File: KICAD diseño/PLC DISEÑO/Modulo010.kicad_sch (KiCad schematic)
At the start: 8 parts

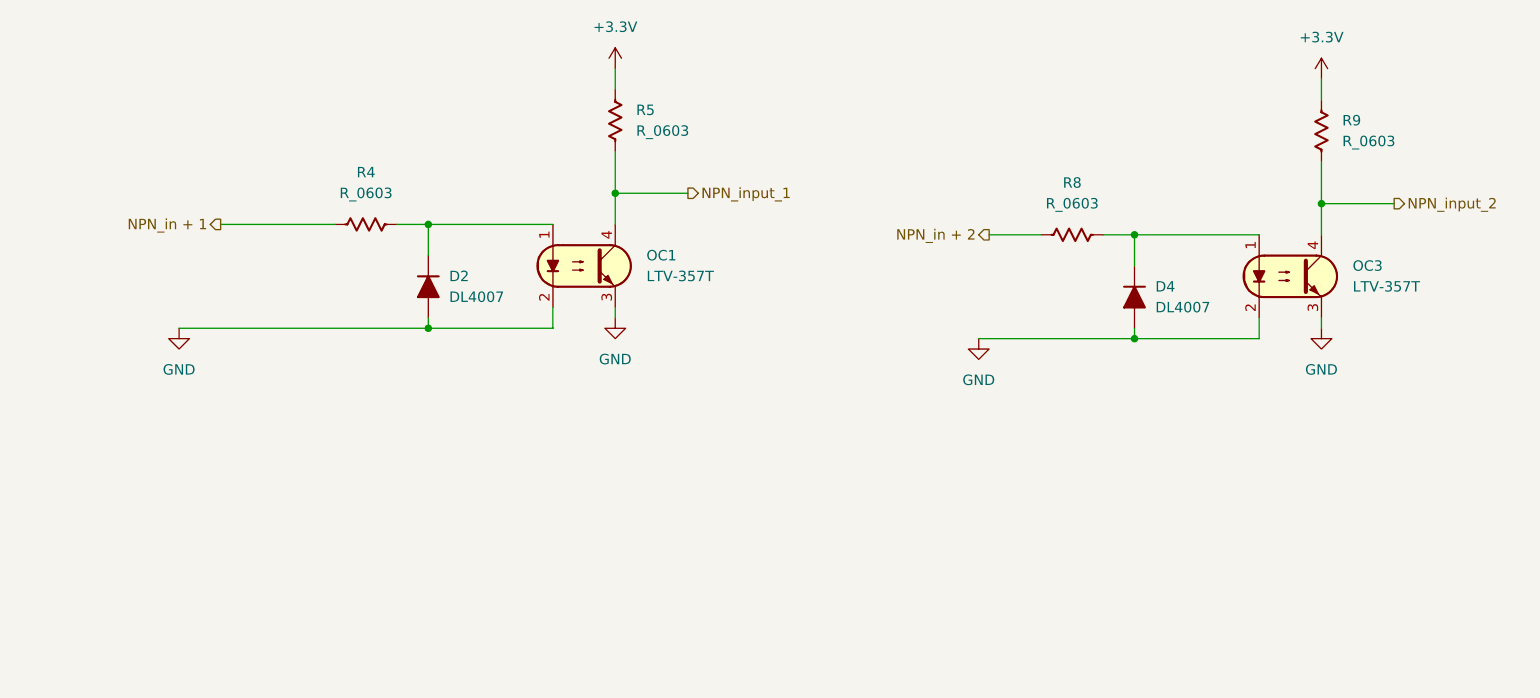
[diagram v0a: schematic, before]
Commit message: Actualizacion estoy cansado jefe :)
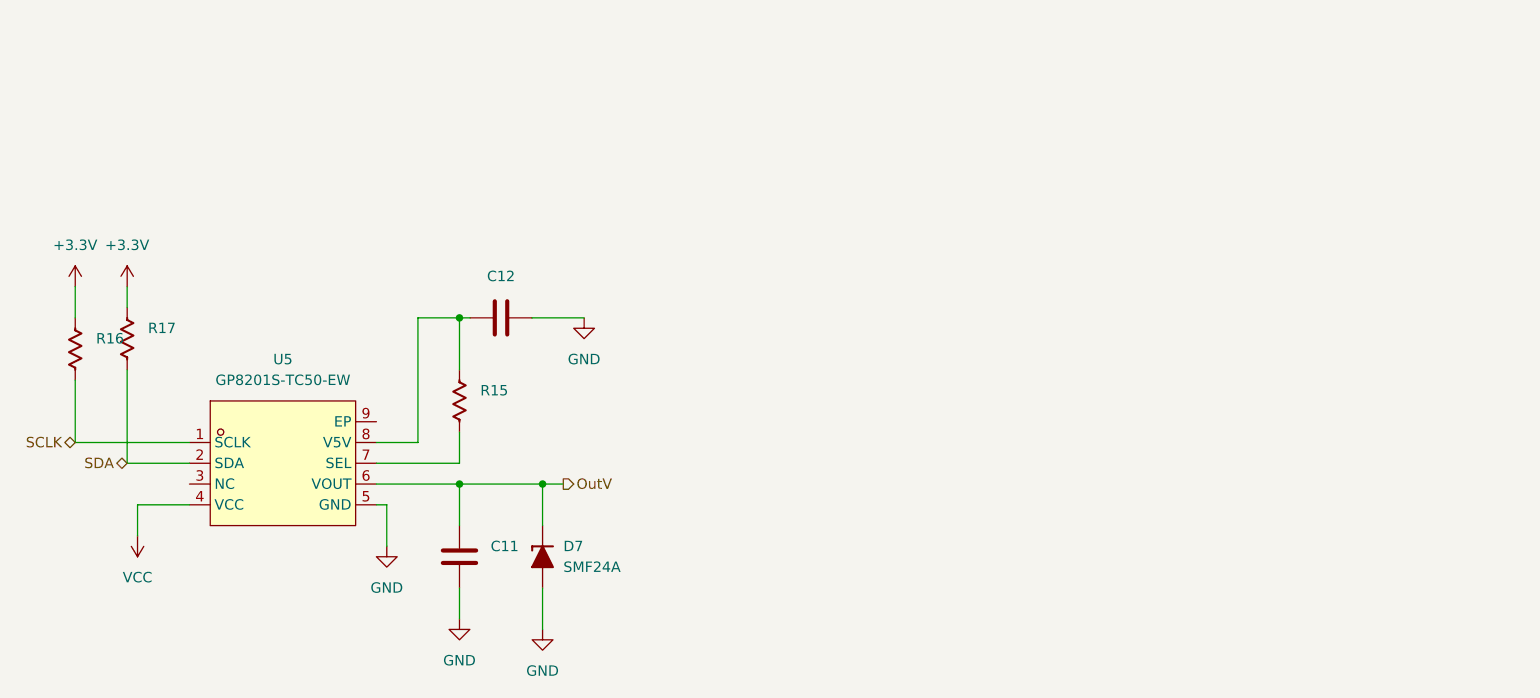
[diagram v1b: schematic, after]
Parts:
- removed D2, D4: DL4007, PCM_Diode_SMD_AKL:D_MELF, symbol PCM_Diode_AKL:DL4007
- removed OC1, OC3: LTV-357T, PCM_Package_SO_AKL:SO-4_4.4x3.9mm_P2.54mm, symbol PCM_Optocoupler_AKL:LTV-357T
- removed R4, R5, R8, R9: R_0603, PCM_Resistor_SMD_AKL:R_0603_1608Metric, symbol PCM_Resistor_US_AKL:R_0603
- added C11, C12: C_0603, PCM_Capacitor_SMD_AKL:C_0603_1608Metric, symbol PCM_Capacitor_AKL:C_0603
- added D7: SMF24A, PCM_Diode_SMD_AKL:D_SOD-123F, symbol PCM_Diode_TVS_AKL:SMF24A
- added R15, R16, R17: R_0603, PCM_Resistor_SMD_AKL:R_0603_1608Metric, symbol PCM_Resistor_US_AKL:R_0603
- added U5: GP8201S-TC50-EW, EasyEDA:ESOP-8_L4.9-W3.9-P1.27-LS6.0-BL-EP, symbol Cris:GP8201S-TC50-EW
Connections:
- net +3.3V: now also R16.1, R17.1
- net GND: now also C11.2, C12.2, D7.2 (A), U5.5 (GND)
- new net: R15.2, U5.7 (SEL)
- new net: C12.1, R15.1, U5.8 (V5V)
- new net OutV: C11.1, D7.1 (K), U5.6 (VOUT)
- new net SCLK: R16.2, U5.1 (SCLK)
- new net SDA: R17.2, U5.2 (SDA)
- new net VCC: U5.4 (VCC)
